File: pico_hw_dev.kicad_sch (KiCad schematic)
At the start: 5 parts

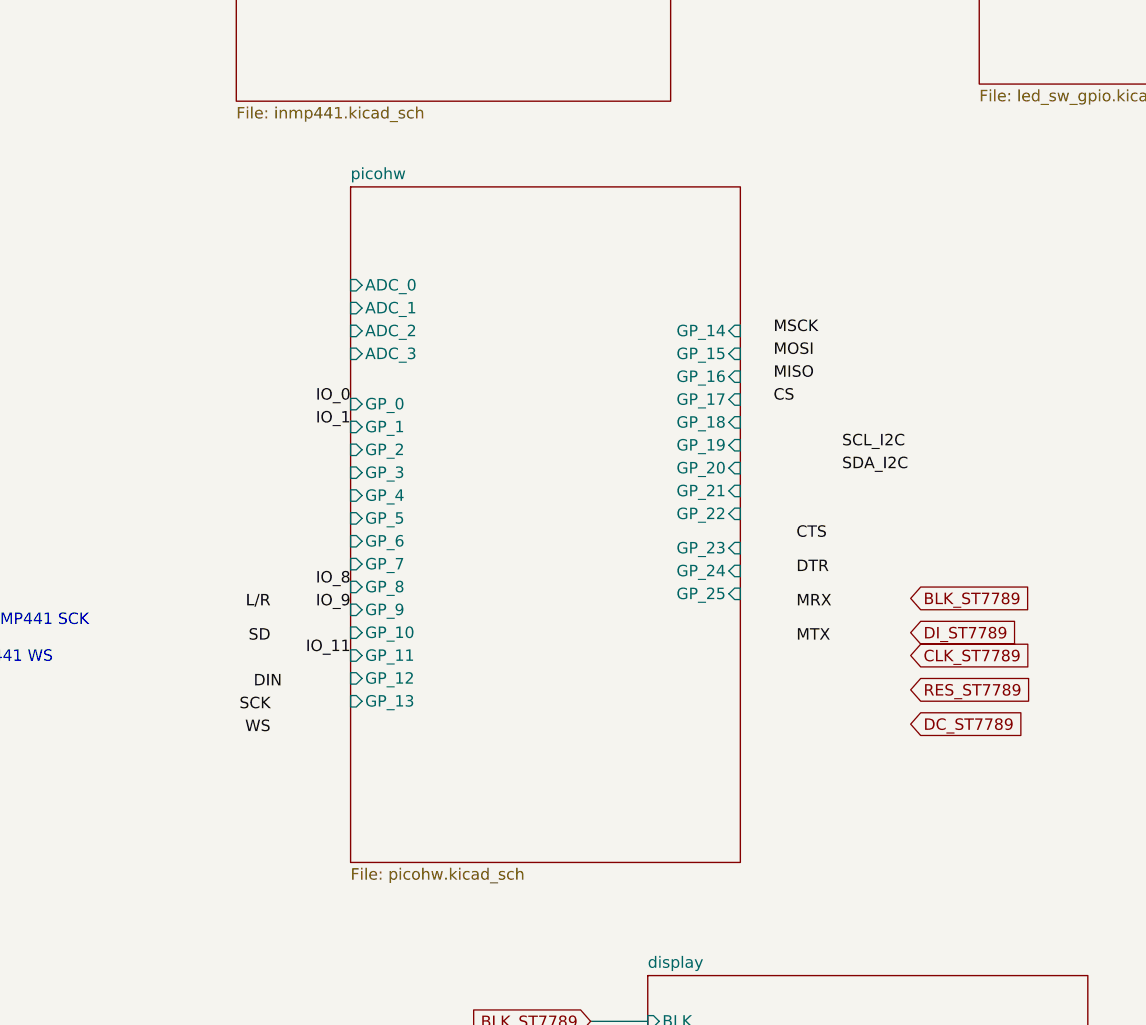
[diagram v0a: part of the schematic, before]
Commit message: Update KiCad project files
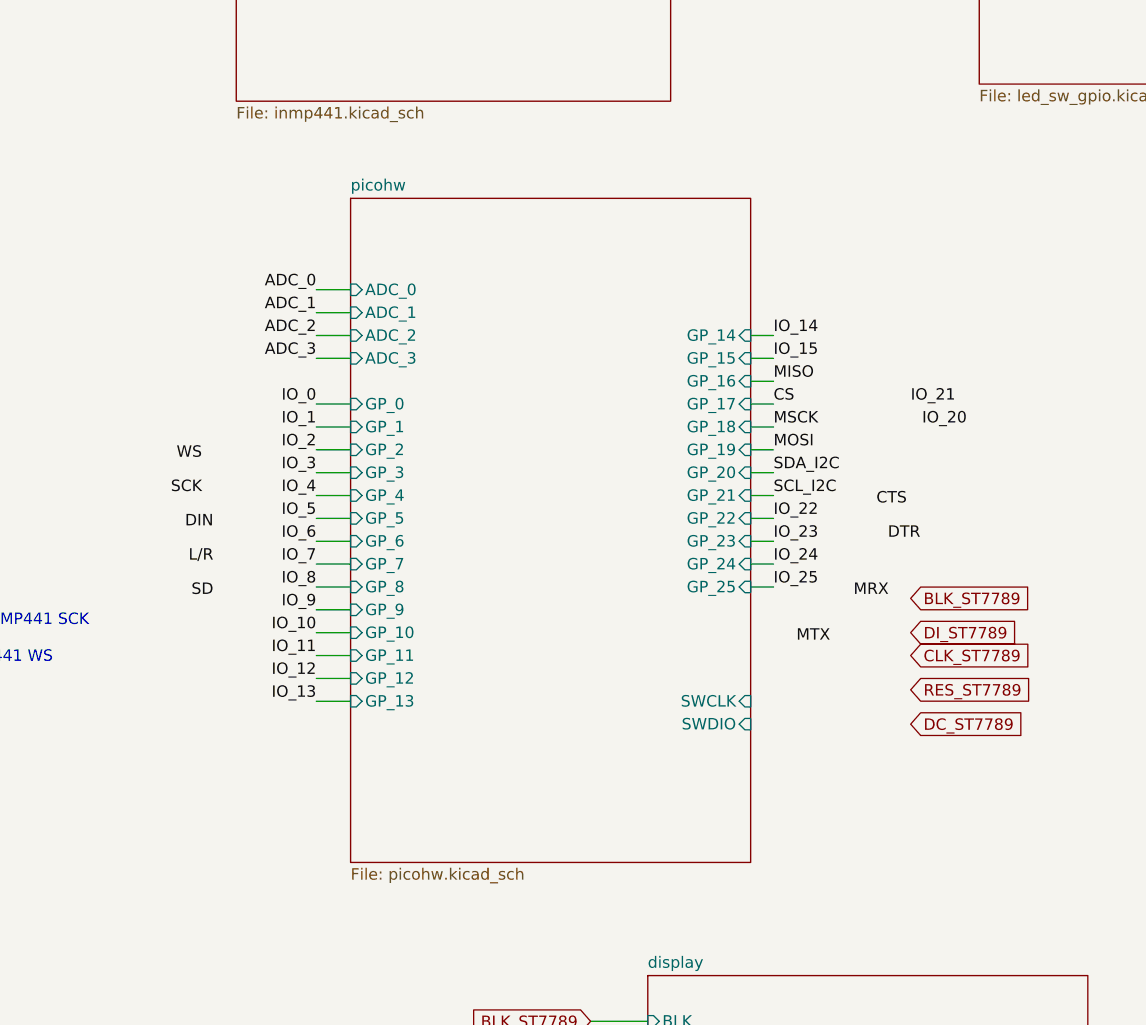
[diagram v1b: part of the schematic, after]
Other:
- sheet picohw ports: added SWCLK, SWDIO; removed none
